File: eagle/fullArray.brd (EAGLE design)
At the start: 29 x 70.1 mm, 115 parts

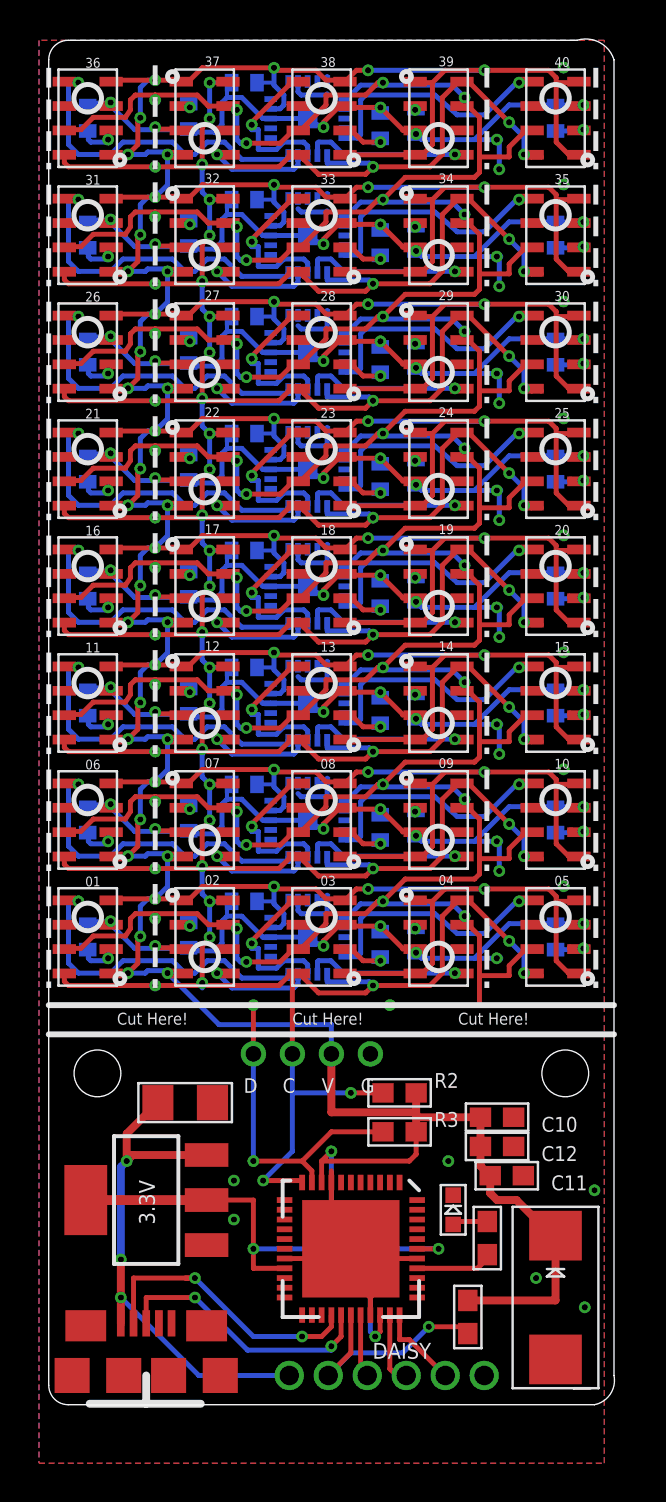
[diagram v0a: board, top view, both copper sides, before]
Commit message: once again, tweak the outline.
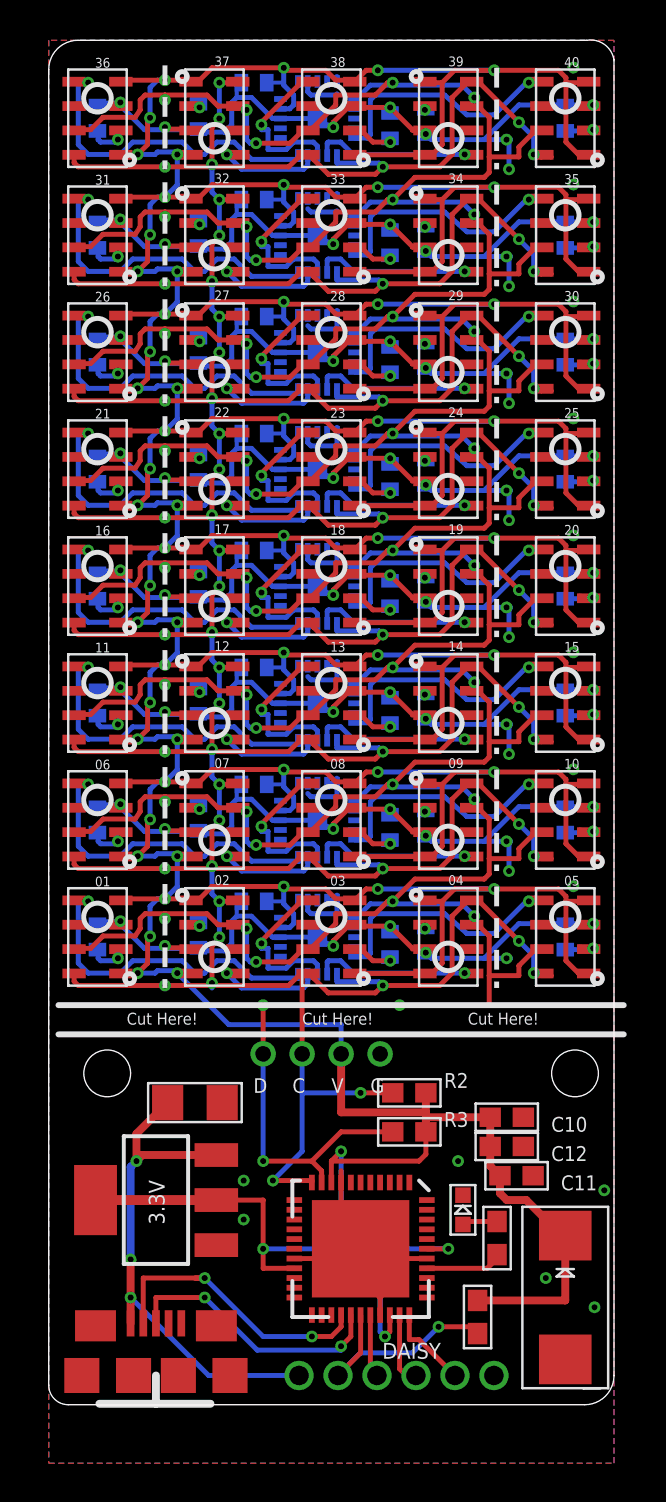
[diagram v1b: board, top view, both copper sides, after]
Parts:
- moved 01 0.50 mm to (2.50, 24.0)
- moved 02 0.50 mm to (8.50, 24.0)
- moved 03 0.50 mm to (14.5, 24.0)
- moved 04 0.50 mm to (20.5, 24.0)
- moved 05 0.50 mm to (26.5, 24.0)
- moved 06 0.50 mm to (2.50, 30.0)
- moved 07 0.50 mm to (8.50, 30.0)
- moved 08 0.50 mm to (14.5, 30.0)
- moved 09 0.50 mm to (20.5, 30.0)
- moved 10 0.50 mm to (26.5, 30.0)
- moved 11 0.50 mm to (2.50, 36.0)
- moved 12 0.50 mm to (8.50, 36.0)
- moved 13 0.50 mm to (14.5, 36.0)
- moved 14 0.50 mm to (20.5, 36.0)
- moved 15 0.50 mm to (26.5, 36.0)
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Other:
- board size 29 x 70.1 mm -> 29 x 70 mm
